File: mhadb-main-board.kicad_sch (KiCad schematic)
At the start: 15 parts, among them U1 ESP32-S3FN8

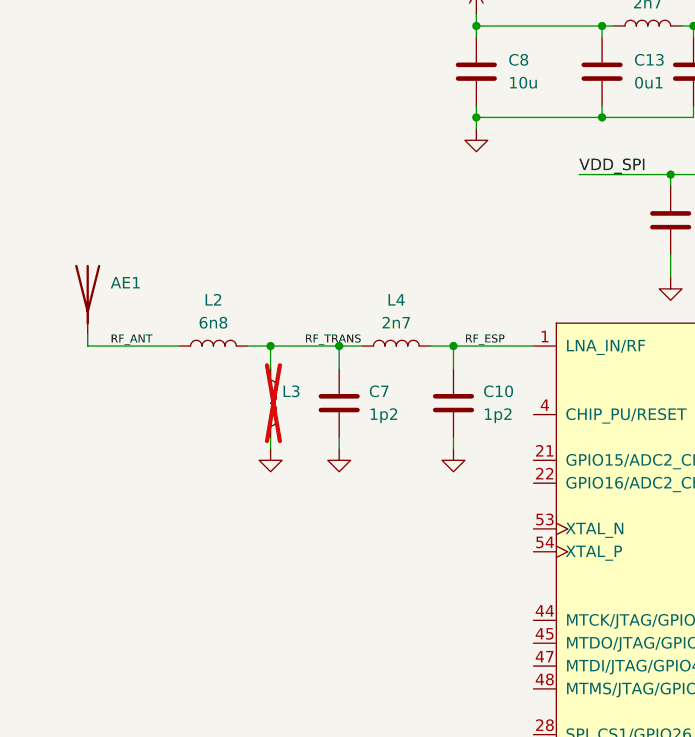
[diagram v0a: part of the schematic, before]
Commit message: schem: import reset circuit
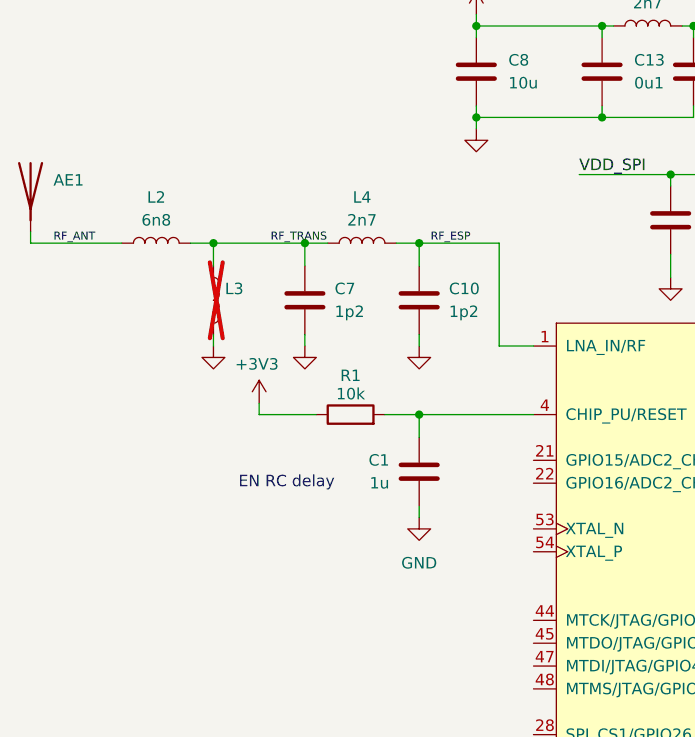
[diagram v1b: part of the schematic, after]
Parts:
- added C1: 1u, Capacitor_SMD:C_0402_1005Metric, symbol Device:C
- added R1: 10k, Resistor_SMD:R_0402_1005Metric, symbol Device:R
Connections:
- net +3V3: now also R1.1
- net GND: now also C1.2
- net at U1.4 (CHIP_PU/RESET): now also C1.1, R1.2
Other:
- note added: "EN RC delay"
- moved on the sheet: AE1, C10, C7, L2, L3, L4
